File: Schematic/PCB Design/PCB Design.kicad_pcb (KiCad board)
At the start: 2 copper layers, 56.6 x 59.2 mm, 12 parts, among them J1 Conn_01x08, J2 Conn_01x01, J3 Conn_01x01, J4 Conn_01x02, J5 Conn_01x08, J6 Conn_01x04, U1 74HC137, U2 ESP32-CAM, U3 74LS151, U5 74LS04, U6 74LS04

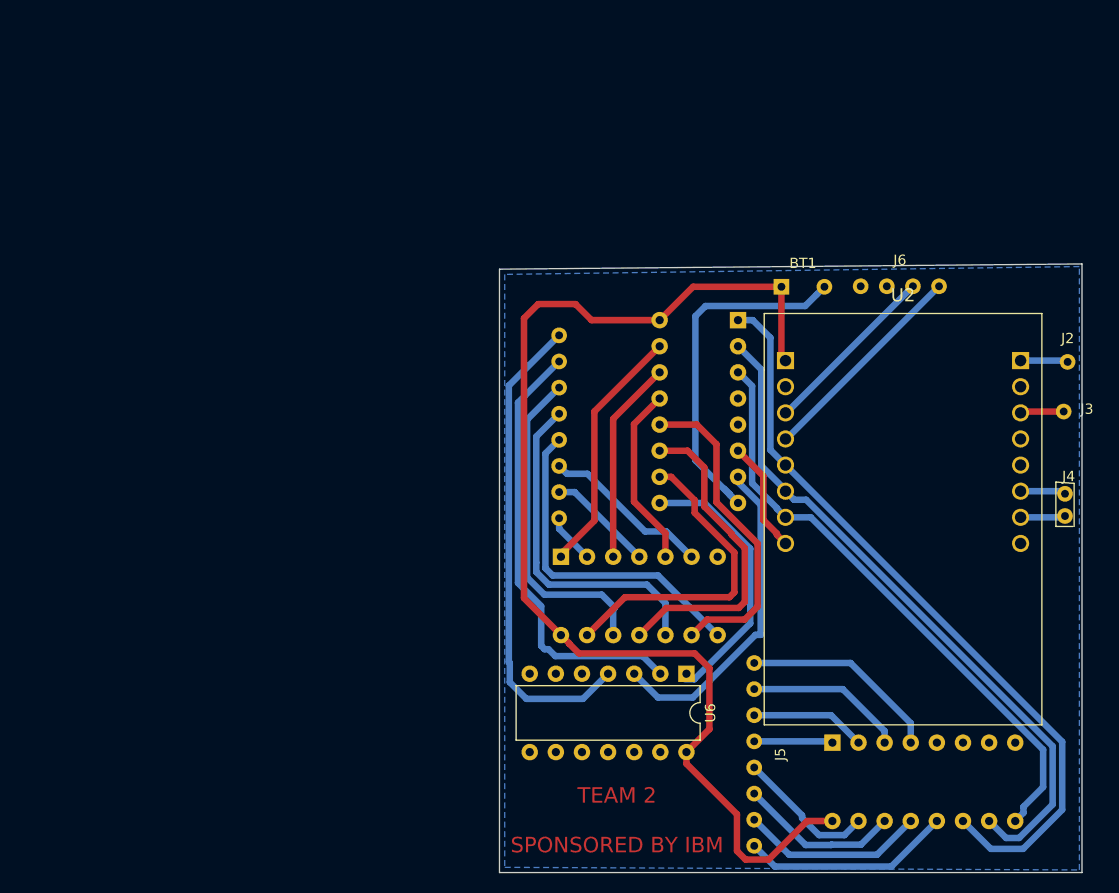
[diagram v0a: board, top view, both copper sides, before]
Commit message: initiated rev 2A of the board design
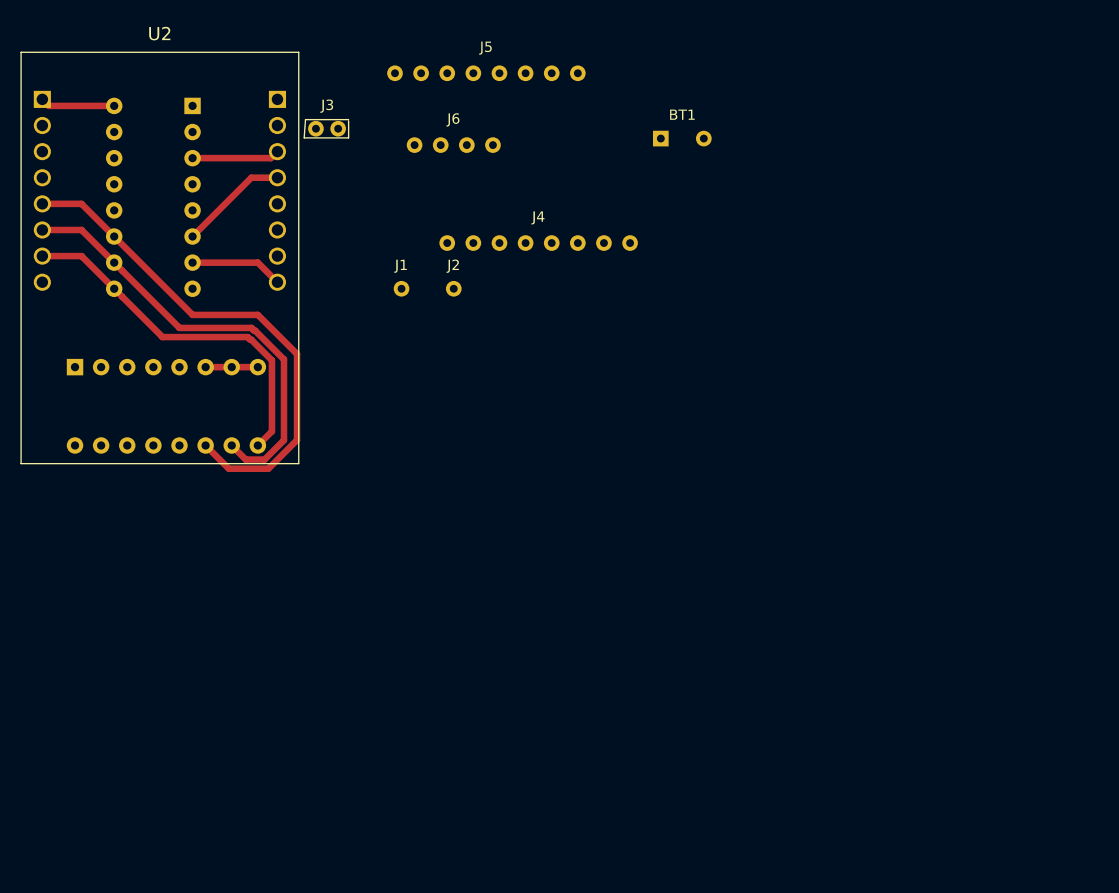
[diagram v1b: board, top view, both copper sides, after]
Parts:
- removed U5, U6: 74LS04, Package_DIP:DIP-14_W7.62mm
- J1: value Conn_01x08 -> DHT11; footprint PCB Design:conn_01x08 -> PCB Design:conn_01x01; moved to F.Cu
- J2: value Conn_01x01 -> 3..3V Out
- J3: value Conn_01x01 -> RX/TX; footprint PCB Design:conn_01x01 -> PCB Design:conn_01x02
- J4: value Conn_01x02 -> TrigSendPins; footprint PCB Design:conn_01x02 -> PCB Design:conn_01x08
- J5: value Conn_01x08 -> EchoReturnPins
- U1: value 74HC137 -> CD4051B
- U3: value 74LS151 -> CD4051B
- moved U3 82.2 mm to (85.7, 95.9)
- moved J3 76.7 mm to (110.3, 72.7)
- moved U2 76.6 mm to (94.0, 83.8)
- moved J5 71.2 mm to (125.7, 67.3), turned to 0 degrees
- moved J2 60.1 mm to (122.6, 88.3)
- moved J4 57.2 mm to (130.8, 83.8), turned to 0 degrees
- moved U1 57.0 mm to (97.2, 70.5)
- moved J6 45.5 mm to (122.6, 74.3)
- moved J1 20.4 mm to (117.5, 88.3), turned to 0 degrees
- moved BT1 18.6 mm to (144.8, 73.7)
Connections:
- net /ESP32-CAM Module/displayCLA renamed /displayCLA
- net /ESP32-CAM Module/displaySDA renamed /displaySDA
- J1 pad 1: /ESP32-CAM Module/Y0 -> Net-(J1-Pad1)
- U1 pad 1: /ESP32-CAM Module/selectA0 -> Net-(J4-Pad5)
- U1 pad 10: /ESP32-CAM Module/~Y5 -> /selectB
- U1 pad 11: /ESP32-CAM Module/~Y4 -> /selectA
- U1 pad 12: /ESP32-CAM Module/~Y3 -> Net-(J4-Pad4)
- U1 pad 13: /ESP32-CAM Module/~Y2 -> Net-(J4-Pad1)
- U1 pad 14: /ESP32-CAM Module/~Y1 -> Net-(J4-Pad2)
- U1 pad 15: /ESP32-CAM Module/~Y0 -> Net-(J4-Pad3)
- U1 pad 2: /ESP32-CAM Module/selectA1 -> Net-(J4-Pad7)
- U1 pad 3: /ESP32-CAM Module/selectA2 -> /enable
- U1 pad 4: GND -> Net-(J4-Pad8)
- U1 pad 5: GND -> Net-(J4-Pad6)
- U1 pad 6: /ESP32-CAM Module/enable -> GND
- U1 pad 7: /ESP32-CAM Module/~Y7 -> GND
- U1 pad 9: /ESP32-CAM Module/~Y6 -> /selectC
- U2 pad 1: /ESP32-CAM Module/enable -> Net-(J1-Pad1)
- U2 pad 10: /ESP32-CAM Module/echoSignal -> /echoSignal
- U2 pad 11: Net-(J3-Pad1) -> /enable
- U2 pad 13: Net-(U2-Pad13) -> (no net)
- U2 pad 14: Net-(J4-Pad1) -> Net-(J3-Pad1)
- U2 pad 15: Net-(J4-Pad2) -> Net-(J3-Pad2)
- U2 pad 2: /ESP32-CAM Module/selectA2 -> /selectC
- U2 pad 3: /ESP32-CAM Module/selectA1 -> /selectB
- U2 pad 4: /ESP32-CAM Module/selectA0 -> /selectA
- U3 pad 1: Net-(J5-Pad4) -> Net-(J5-Pad5)
- U3 pad 10: /ESP32-CAM Module/selectA1 -> /selectB
- U3 pad 11: /ESP32-CAM Module/selectA0 -> /selectA
- U3 pad 12: Net-(J5-Pad8) -> Net-(J5-Pad4)
- U3 pad 13: Net-(J5-Pad7) -> Net-(J5-Pad1)
- U3 pad 14: Net-(J5-Pad6) -> Net-(J5-Pad2)
- U3 pad 15: Net-(J5-Pad5) -> Net-(J5-Pad3)
- U3 pad 2: Net-(J5-Pad3) -> Net-(J5-Pad7)
- U3 pad 3: Net-(J5-Pad2) -> /echoSignal
- U3 pad 4: Net-(J5-Pad1) -> Net-(J5-Pad8)
- U3 pad 5: /ESP32-CAM Module/echoSignal -> Net-(J5-Pad6)
- U3 pad 6: Net-(U3-Pad6) -> GND
- U3 pad 9: /ESP32-CAM Module/selectA2 -> /selectC
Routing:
- net +5V: track 114.9 -> 7.25 mm
- net /ESP32-CAM Module/selectA0: track 73.9 -> 0.00 mm
- net /ESP32-CAM Module/selectA1: track 66.1 -> 0.00 mm
- net /ESP32-CAM Module/selectA2: track 58.5 -> 0.00 mm
- net /selectA: track 0.00 -> 50.2 mm
- net /ESP32-CAM Module/Y7: track 47.0 -> 0.00 mm
- net /selectB: track 0.00 -> 43.0 mm
- net /ESP32-CAM Module/Y6: track 43.0 -> 0.00 mm
- net /selectC: track 0.00 -> 35.4 mm
- net /ESP32-CAM Module/Y4: track 33.2 -> 0.00 mm
- net /ESP32-CAM Module/Y3: track 32.5 -> 0.00 mm
- net /ESP32-CAM Module/Y5: track 32.2 -> 0.00 mm
- net /ESP32-CAM Module/~Y7: track 32.1 -> 0.00 mm
- net /ESP32-CAM Module/~Y3: track 31.3 -> 0.00 mm
- net /ESP32-CAM Module/~Y4: track 31.3 -> 0.00 mm
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- removed copper zone on B.Cu, net GND
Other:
- board outline removed
- board text removed: "TEAM 2 SPONSORED BY IBM"
